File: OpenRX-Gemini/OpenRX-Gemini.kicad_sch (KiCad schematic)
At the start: 0 parts

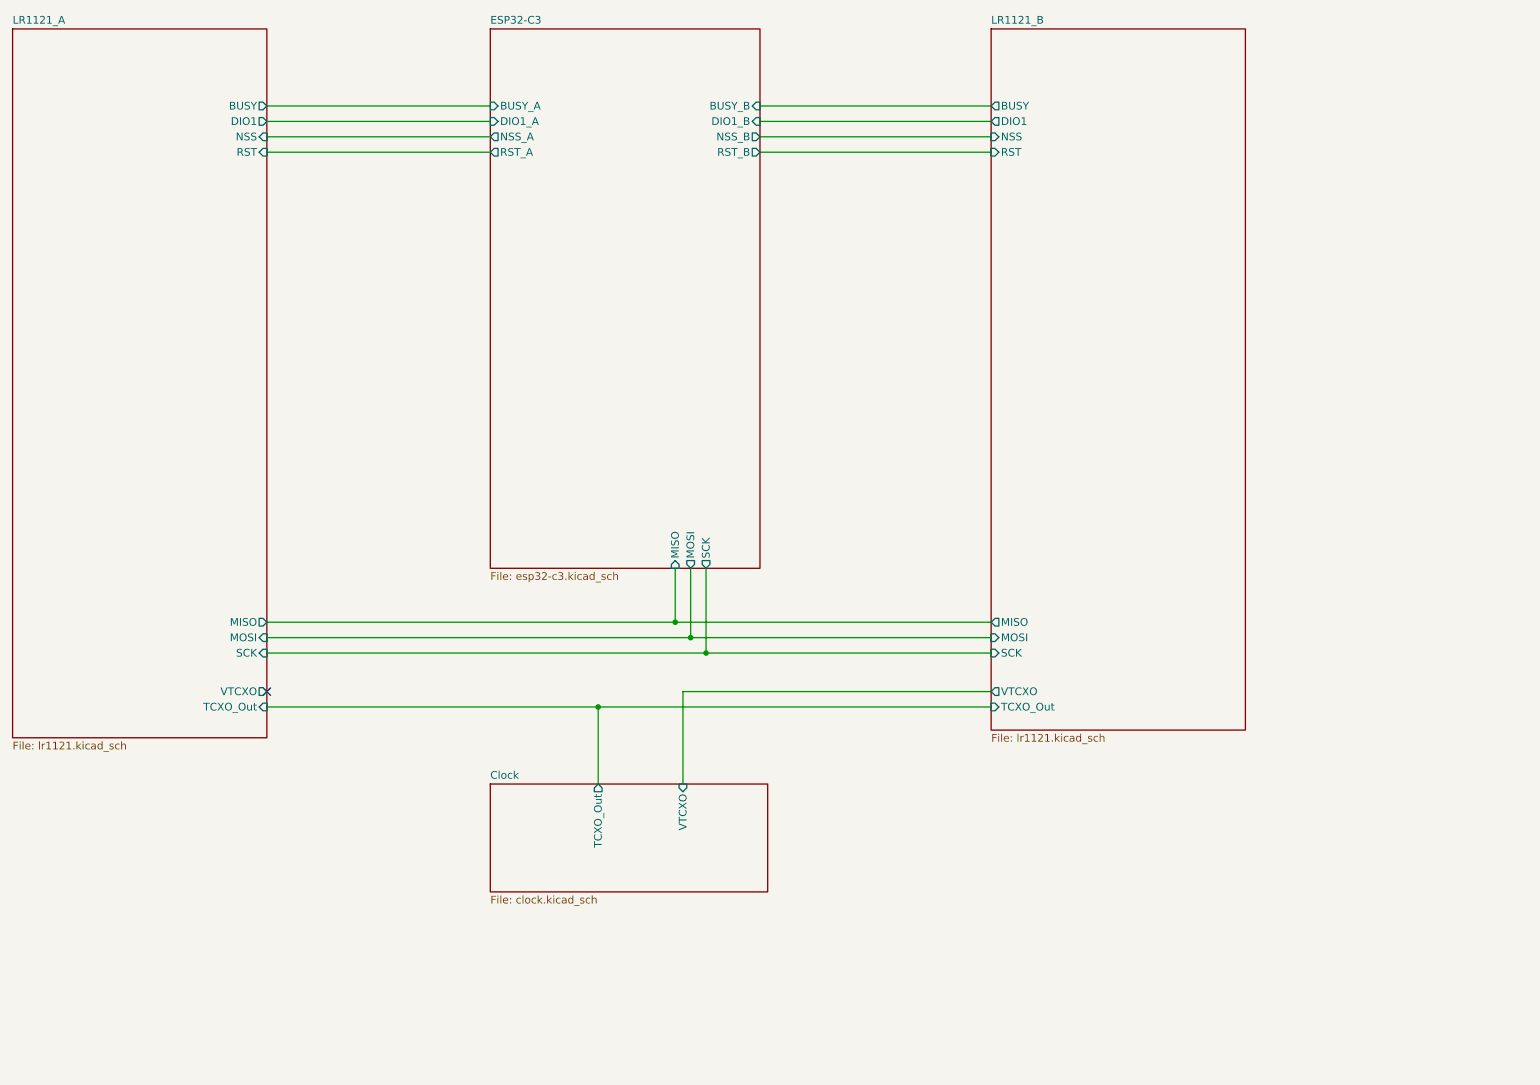
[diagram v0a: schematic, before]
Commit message: annotate
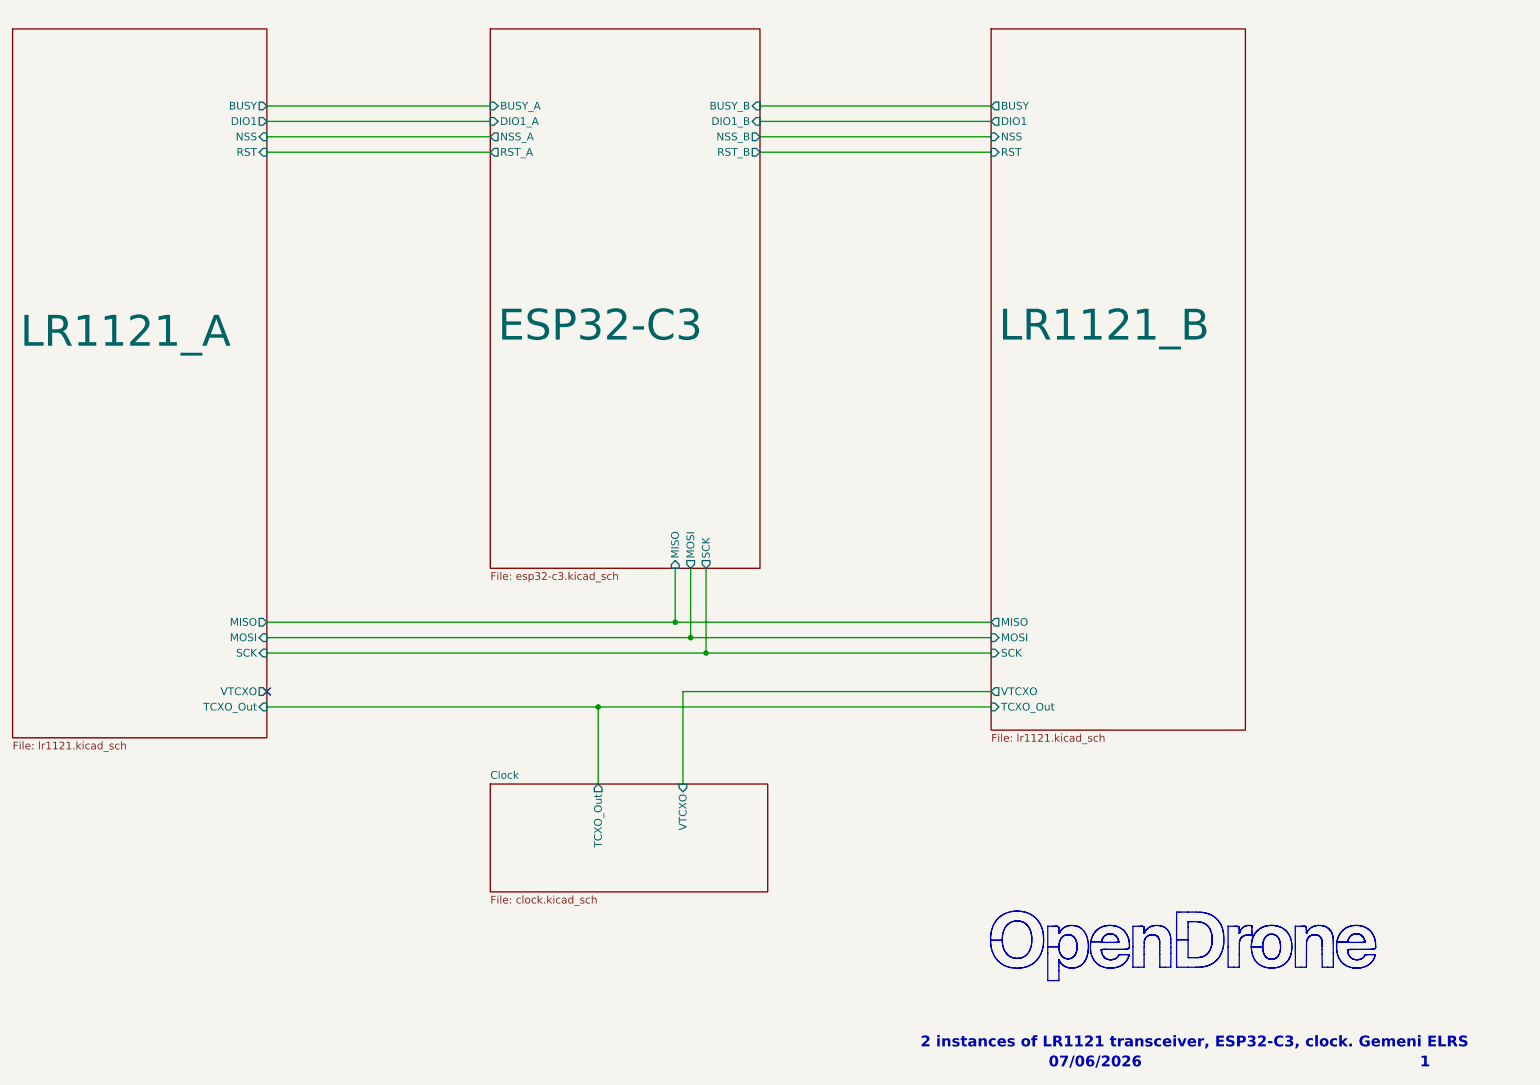
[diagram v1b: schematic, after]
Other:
- note added: "07/06/2026"
- note added: "1"
- note added: "2 instances of LR1121 transceiver, ESP32-C3, clock. Gemeni ELRS"
